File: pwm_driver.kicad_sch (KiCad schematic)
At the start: 16 parts, among them U11 SN74HCS08PWR, U9 SN74HCS02PWR

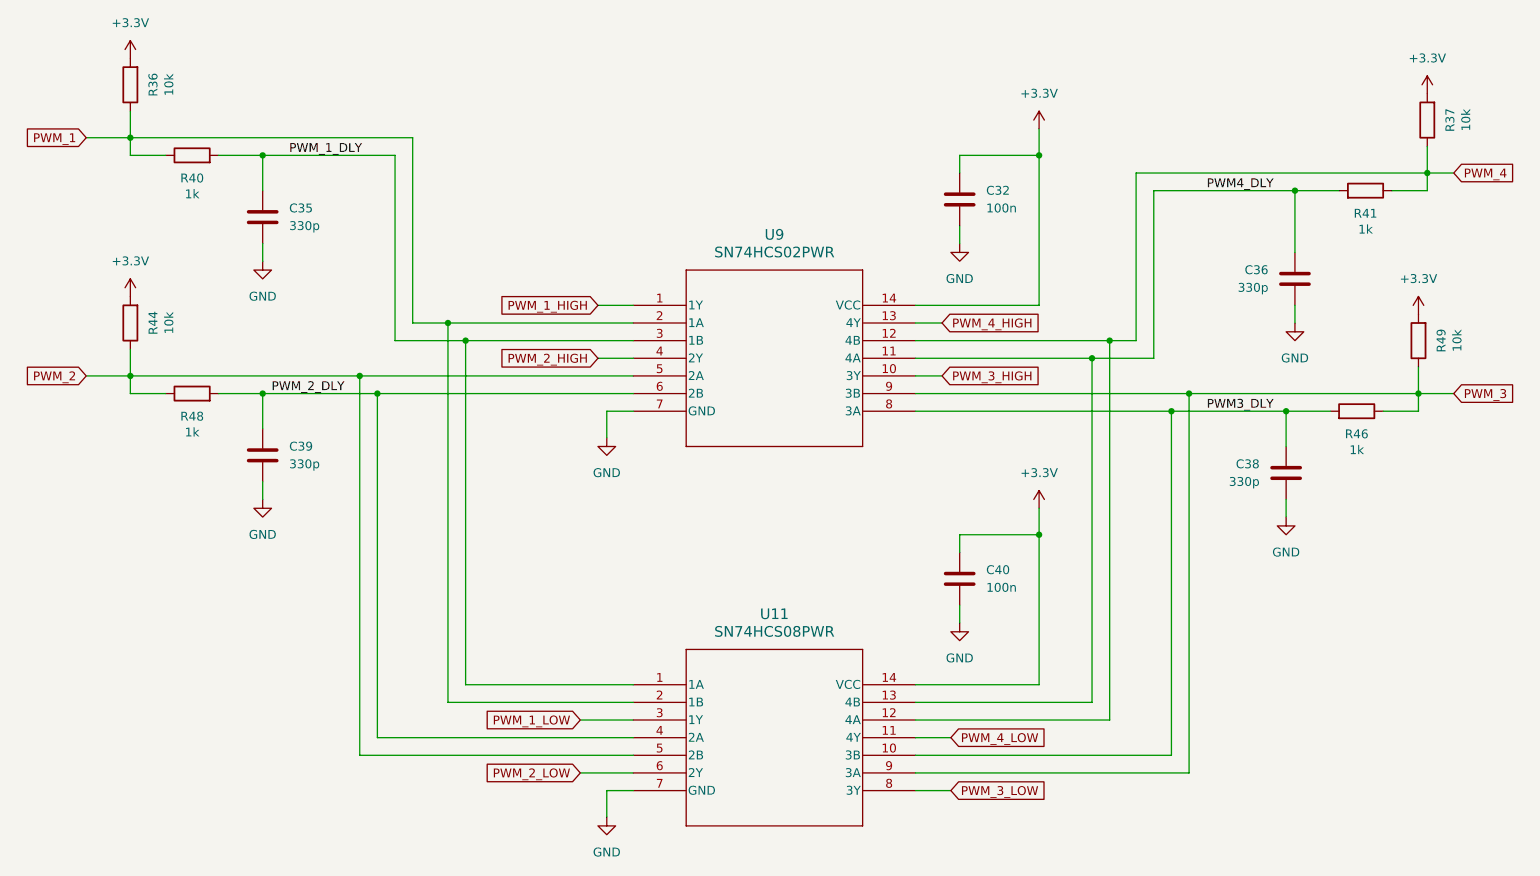
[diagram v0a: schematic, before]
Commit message: generated production files
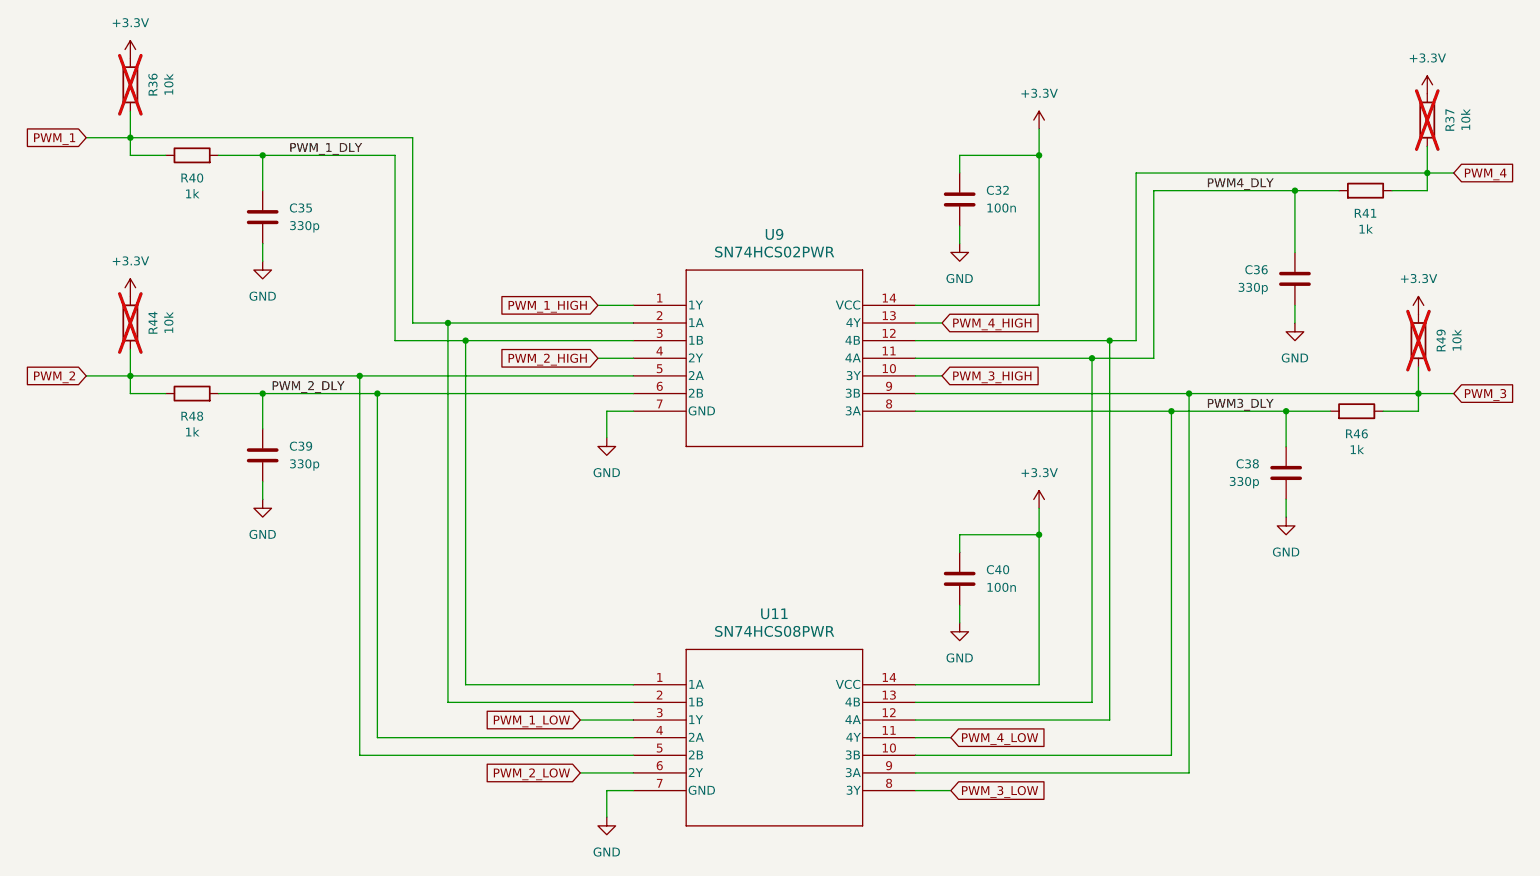
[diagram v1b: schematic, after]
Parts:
- R36, R37, R44, R49: now not fitted
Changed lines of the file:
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@@
 		(on_board yes)
 		(in_pos_files yes)
-		(dnp no)
+		(dnp yes)
 		(property "Reference" "R49"
 			(at 240.792 80.01 90)
@@
 		(on_board yes)
 		(in_pos_files yes)
-		(dnp no)
+		(dnp yes)
 		(property "Reference" "R36"
 			(at 55.372 43.18 90)
@@
 		(on_board yes)
 		(in_pos_files yes)
-		(dnp no)
+		(dnp yes)
 		(property "Reference" "R37"
 			(at 242.062 48.26 90)
@@
 		(on_board yes)
 		(in_pos_files yes)
-		(dnp no)
+		(dnp yes)
 		(property "Reference" "R44"
 			(at 55.372 77.47 90)

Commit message: Fixed DNP parts on BOM
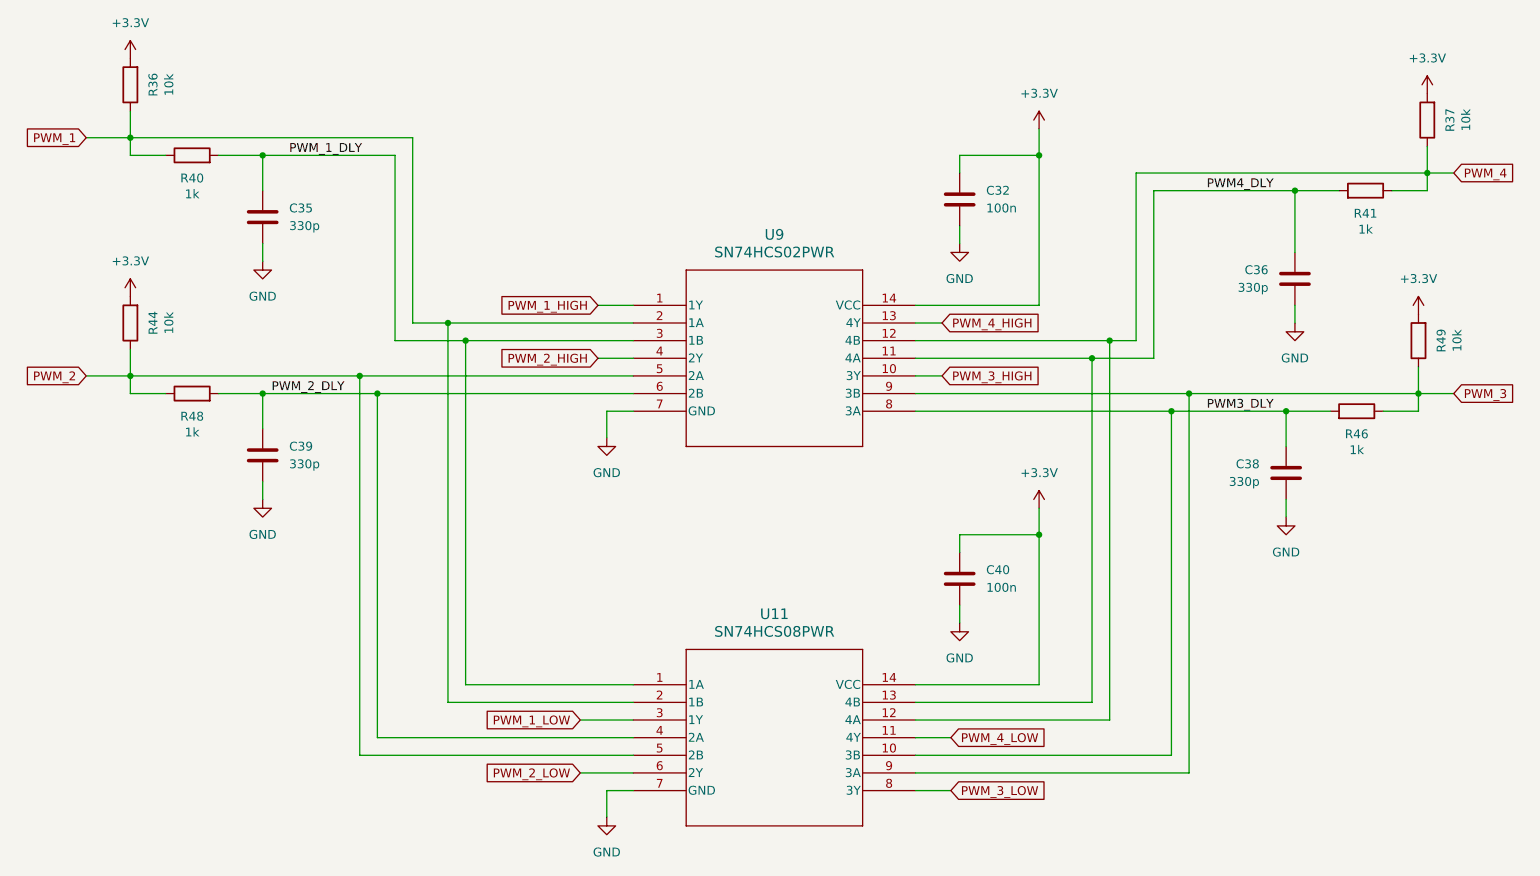
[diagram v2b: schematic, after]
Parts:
- R36, R37, R44, R49: now fitted
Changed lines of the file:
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@@
 		(on_board yes)
 		(in_pos_files yes)
-		(dnp yes)
+		(dnp no)
 		(property "Reference" "R49"
 			(at 240.792 80.01 90)
@@
 		(on_board yes)
 		(in_pos_files yes)
-		(dnp yes)
+		(dnp no)
 		(property "Reference" "R36"
 			(at 55.372 43.18 90)
@@
 		(on_board yes)
 		(in_pos_files yes)
-		(dnp yes)
+		(dnp no)
 		(property "Reference" "R37"
 			(at 242.062 48.26 90)
@@
 		(on_board yes)
 		(in_pos_files yes)
-		(dnp yes)
+		(dnp no)
 		(property "Reference" "R44"
 			(at 55.372 77.47 90)
